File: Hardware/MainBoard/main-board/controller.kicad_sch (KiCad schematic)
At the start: 42 parts, among them J11 Conn_01x04, J12 Conn_01x05, J13 Conn_01x04, J14 Conn_01x06, J15 Conn_01x08, J6 Conn_01x07, J7 Conn_01x04, J8 Conn_01x02, J9 Conn_01x02, Q1 IRLML6244TRPBF, Q2 IRLML6244TRPBF, Q3 IRLML6244TRPBF, Q4 IRLML6244TRPBF, SW2 SW_SPDT, U4 STM32F401RETx, Y2 ATS08A-E

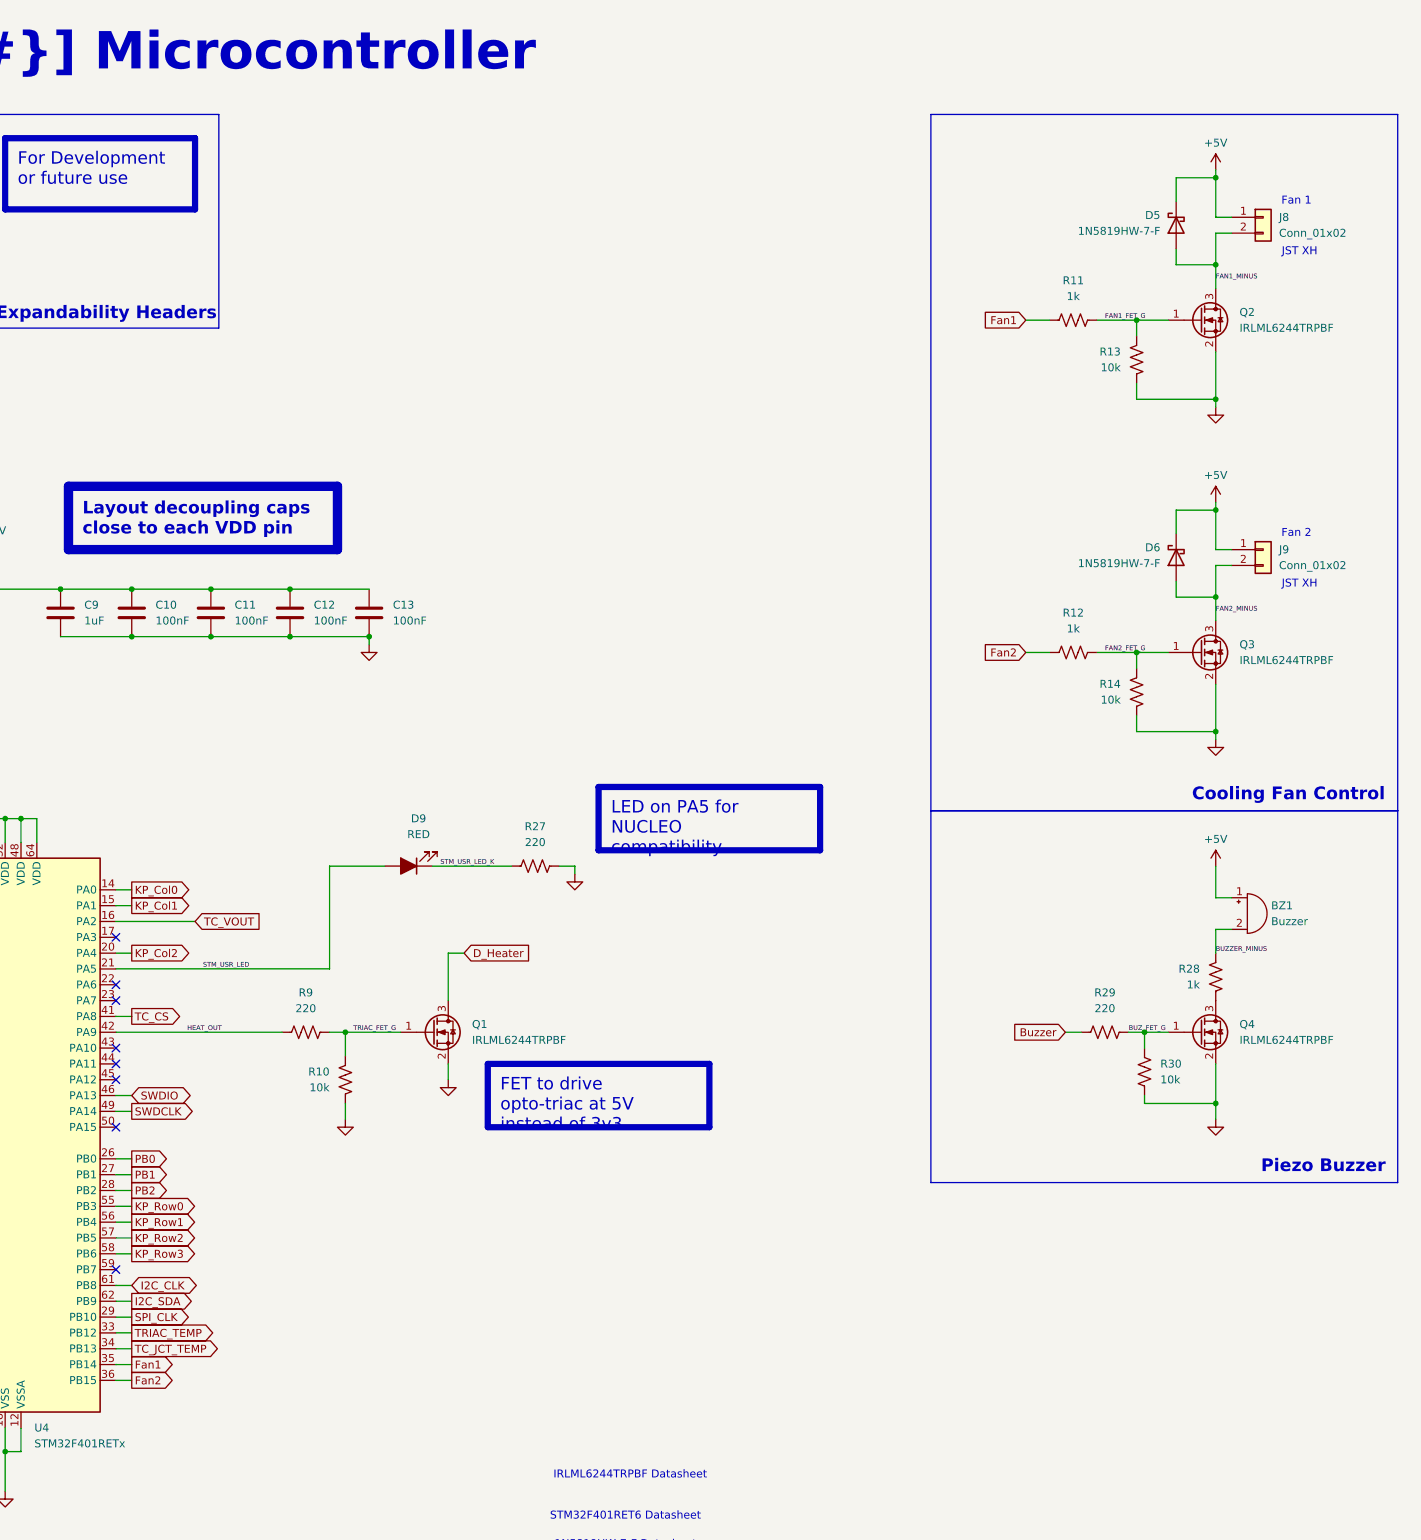
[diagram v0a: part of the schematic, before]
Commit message: working on PCB layout
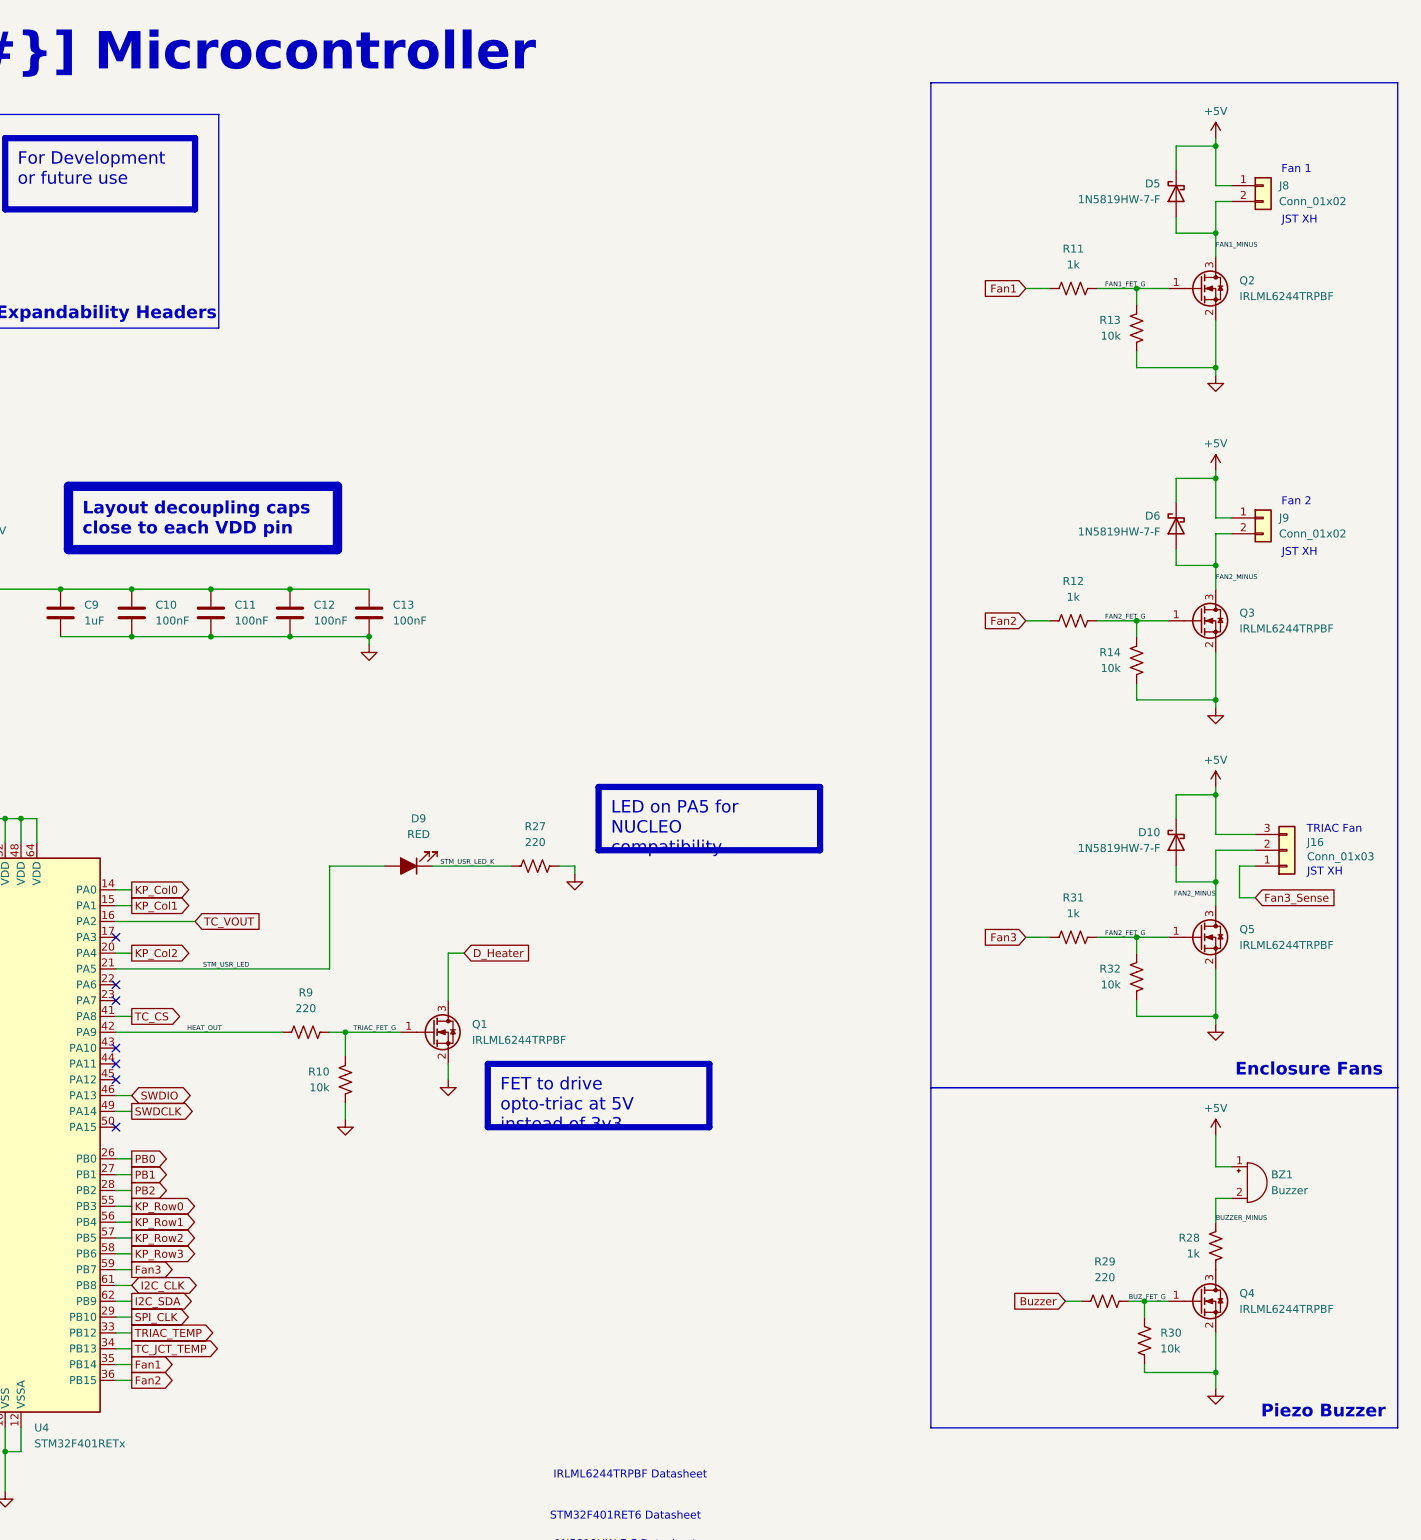
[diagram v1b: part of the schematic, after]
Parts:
- added D10: 1N5819HW-7-F, Diode_SMD:D_SOD-123, symbol Diode:1N5819
- added J16: Conn_01x03, Connector_JST:JST_XH_B3B-XH-A_1x03_P2.50mm_Vertical, symbol Connector_Generic:Conn_01x03
- added Q5: IRLML6244TRPBF, Package_TO_SOT_SMD:SOT-23, symbol Transistor_FET:IRLML6244
- added R31: 1k, Resistor_SMD:R_0603_1608Metric_Pad0.98x0.95mm_HandSolder, symbol Device:R_US
- added R32: 10k, Resistor_SMD:R_0603_1608Metric_Pad0.98x0.95mm_HandSolder, symbol Device:R_US
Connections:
- net +5V: now also D10.1 (K), J16.3 (Pin_3)
- net FAN2_FET_G: now also Q5.1 (G), R31.2, R32.1
- net FAN2_MINUS: now also D10.2 (A), J16.2 (Pin_2), Q5.3 (D)
- net GND: now also Q5.2 (S), R32.2
- net Fan3: now reaches U4.59 (PB7)
- net Fan3: now also R31.1
- new net Fan3_Sense: J16.1 (Pin_1)
- no-connect marks 17 -> 16
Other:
- note added: "Enclosure Fans"
- note added: "TRIAC Fan"
- note removed: "Cooling Fan Control"
- moved on the sheet: BZ1, D5, D6, J8, J9, Q2, Q3, Q4, R11, R12, R13, R14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
